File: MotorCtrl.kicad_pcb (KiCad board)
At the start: 2 copper layers, 47 x 52.1 mm, 10 parts, among them J1 Conn_01x03_Female, J2 Conn_01x02_Female, J3 Conn_01x02_Female, Q1 BS108, Q2 IRLB8721PBF

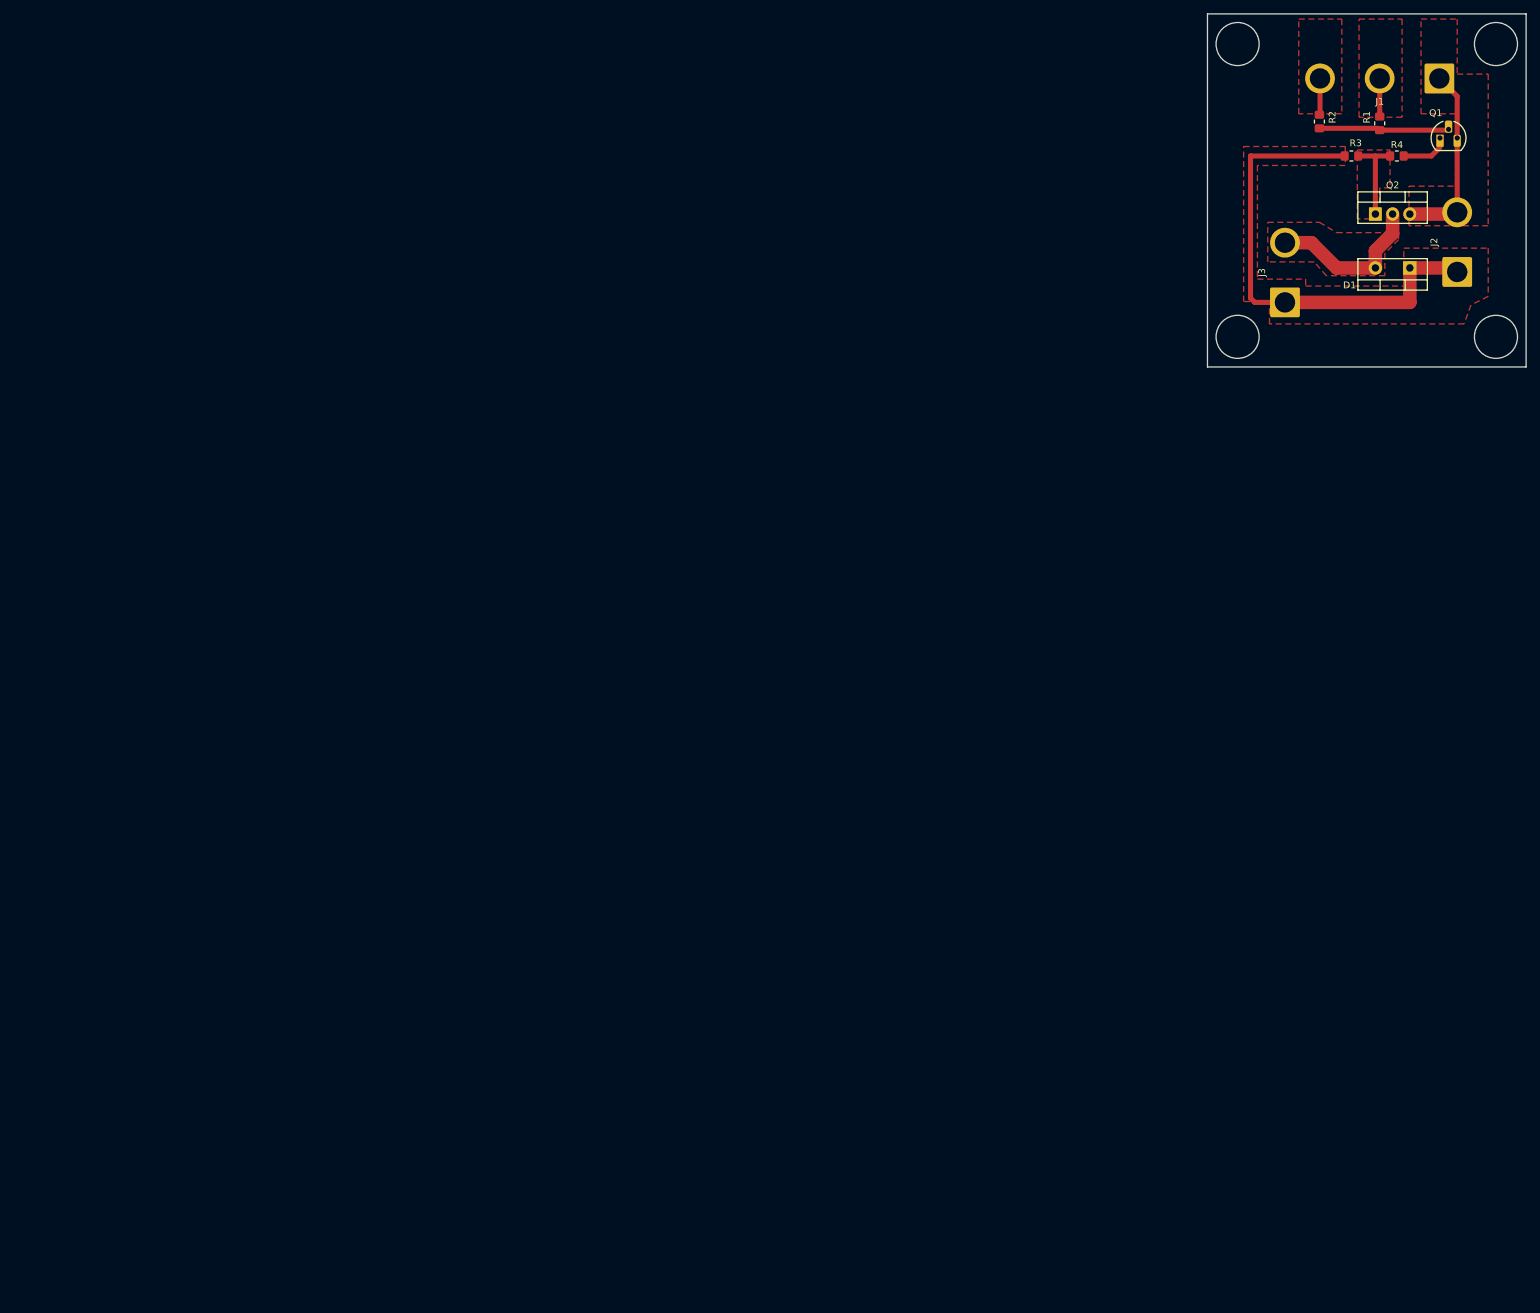
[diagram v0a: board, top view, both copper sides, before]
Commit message: ff
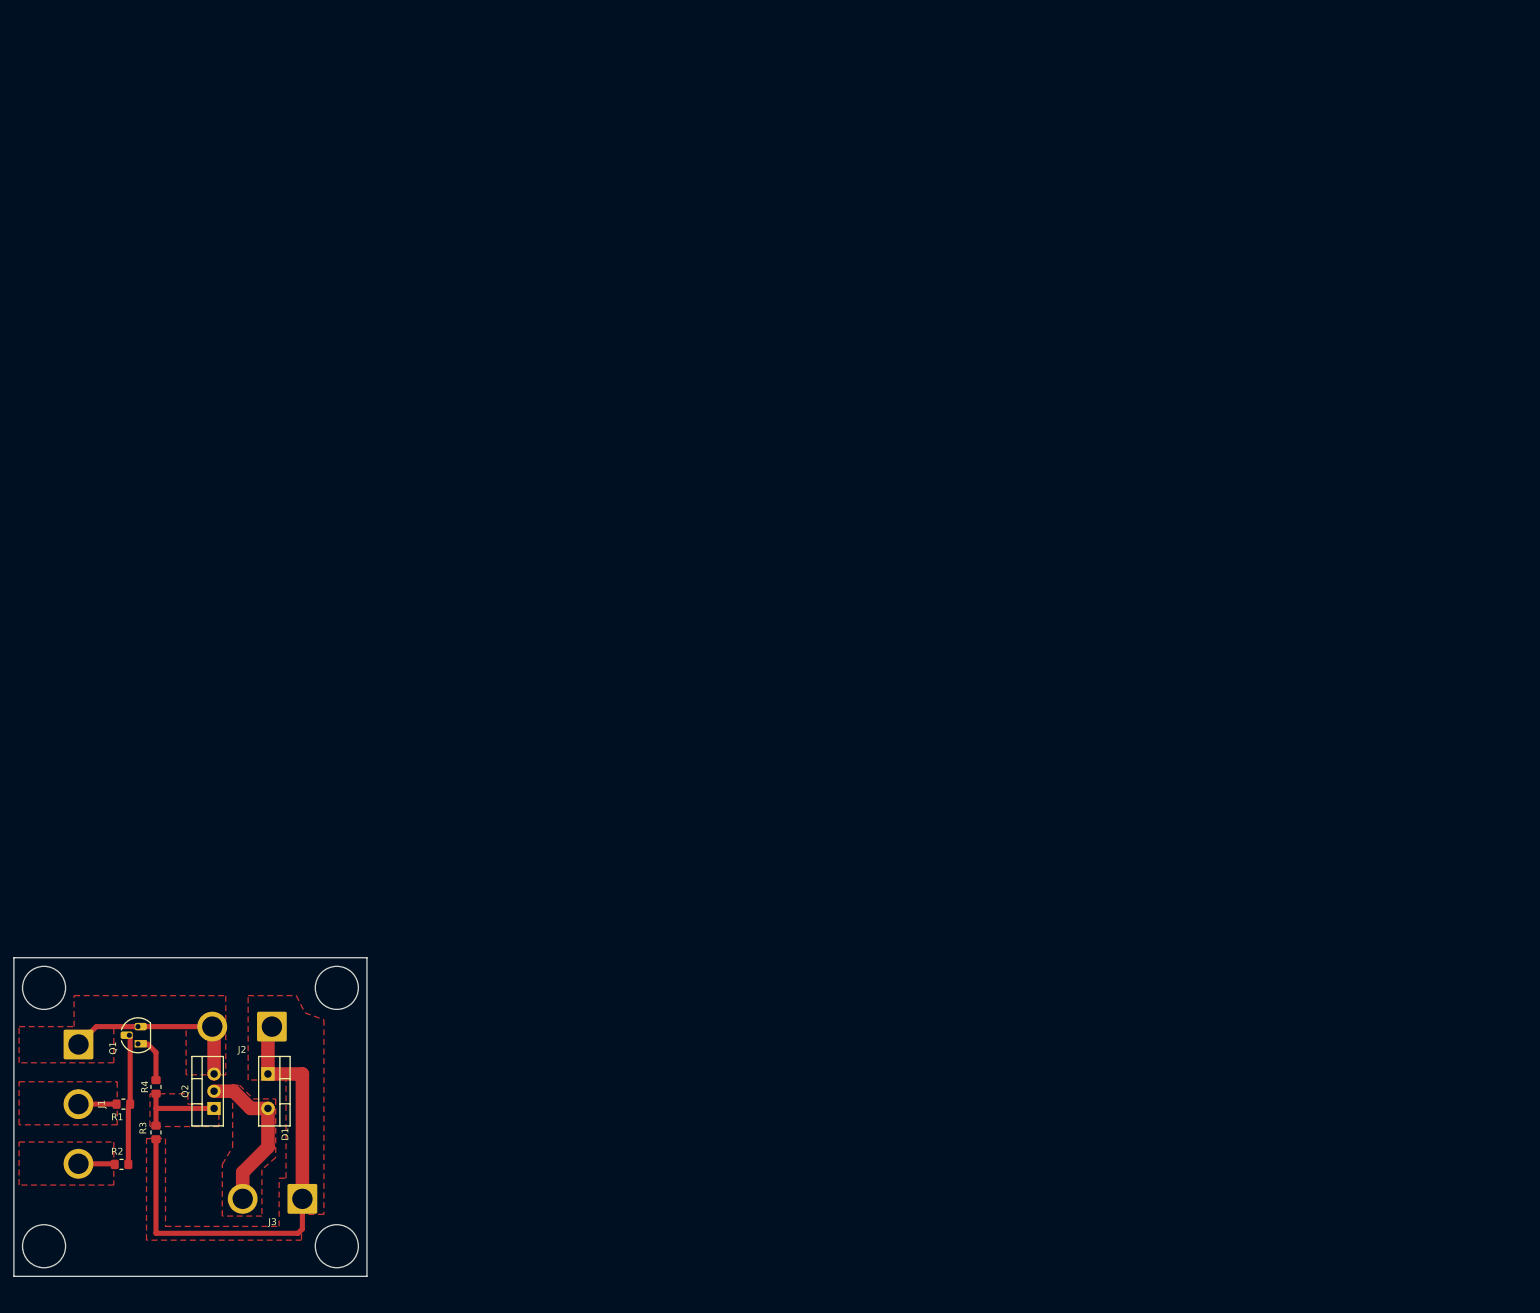
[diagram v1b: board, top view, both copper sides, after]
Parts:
- moved J1 246.1 mm to (25.3, 248.5), turned to -90 degrees
- moved R1 235.0 mm to (31.9, 257.3), turned to 180 degrees
- moved R2 234.2 mm to (31.6, 266.2), turned to 0 degrees
- moved Q1 233.9 mm to (34.0, 248.4), turned to 90 degrees
- moved R4 228.8 mm to (36.7, 254.8), turned to 90 degrees
- moved R3 227.6 mm to (36.7, 261.5), turned to 90 degrees
- moved Q2 216.2 mm to (45.3, 257.9), turned to 90 degrees
- moved J2 207.2 mm to (53.8, 245.9), turned to 180 degrees
- moved D1 206.1 mm to (53.2, 252.9), turned to -90 degrees
- moved J3 196.2 mm to (58.3, 271.3), turned to 180 degrees
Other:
- board size 47 x 52.1 mm -> 52.1 x 47 mm

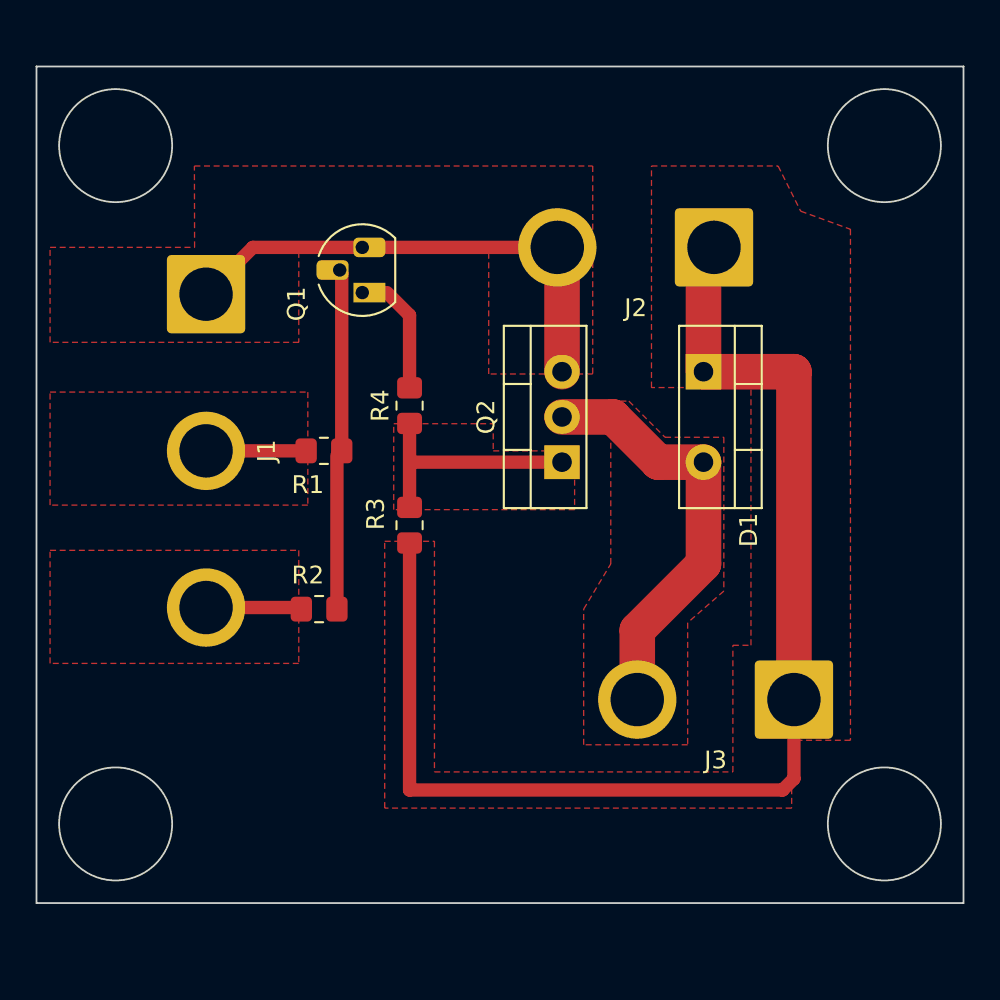
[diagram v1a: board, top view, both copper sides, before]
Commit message: round
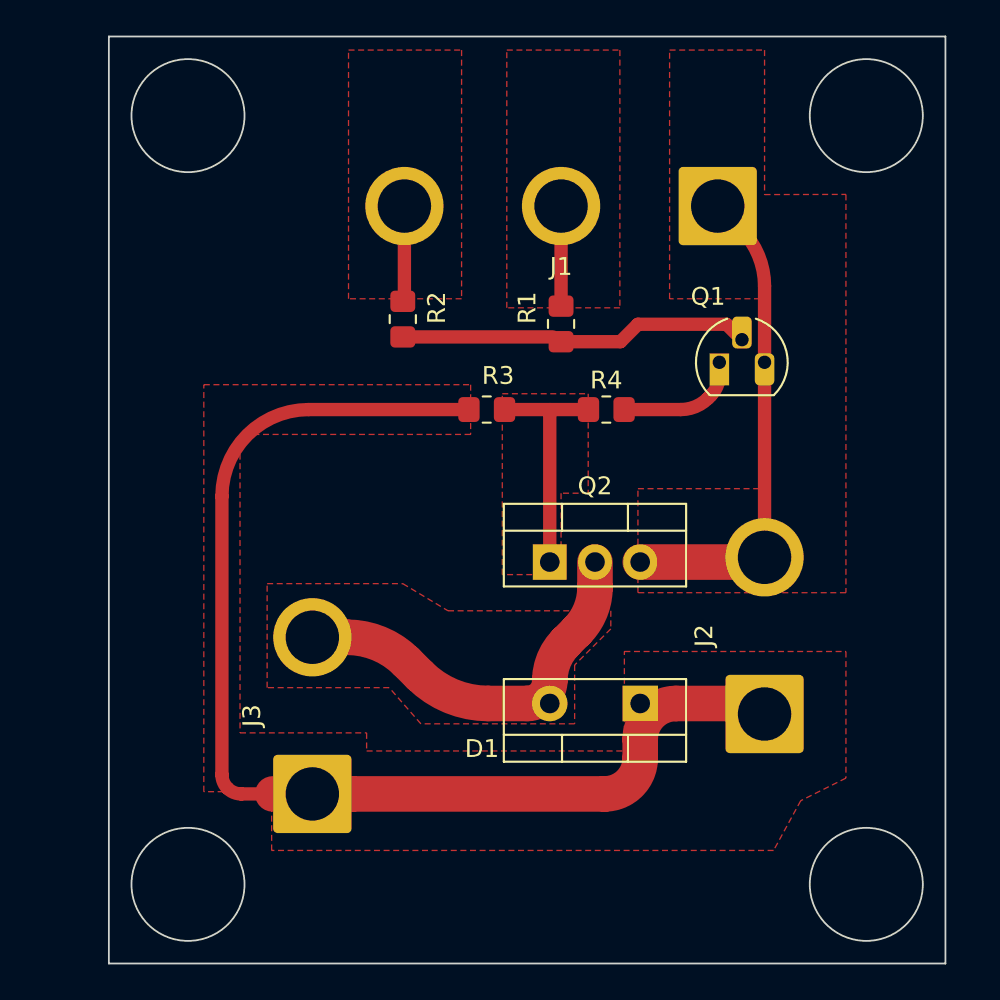
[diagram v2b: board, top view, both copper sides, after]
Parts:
- moved J1 29.2 mm to (54.0, 243.6), turned to 180 degrees
- moved J3 27.6 mm to (31.2, 276.6), turned to 90 degrees
- moved J2 26.4 mm to (56.6, 272.1), turned to 90 degrees
- moved Q1 20.4 mm to (54.1, 252.3), turned to 0 degrees
- moved D1 19.0 mm to (49.7, 271.5), turned to 180 degrees
- moved R2 17.0 mm to (36.3, 249.9), turned to -90 degrees
- moved R1 15.1 mm to (45.2, 250.2), turned to 90 degrees
- moved R4 11.1 mm to (47.8, 255.0), turned to 0 degrees
- moved R3 7.81 mm to (41.0, 255.0), turned to 0 degrees
- moved Q2 5.65 mm to (44.6, 263.5), turned to 0 degrees
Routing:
- net +12V: track 71.5 -> 67.2 mm
- net Net-(D1-Pad2): track 23.9 -> 22.5 mm
- net Net-(Q1-Pad2): track 19.2 -> 20.1 mm
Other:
- board size 52.1 x 47 mm -> 47 x 52.1 mm
